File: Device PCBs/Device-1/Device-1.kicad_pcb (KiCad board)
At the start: 2 copper layers, 55 x 55 mm, 61 parts, among them J1 Conn_01x04_Female, J2 Conn_01x04_Female, U1 EBYTE_E32-433T20D, U10 signle_via, U11 signle_via, U12 signle_via, U13 signle_via, U14 signle_via, U15 signle_via, U16 signle_via, U17 signle_via, U18 signle_via, U19 signle_via, U2 MAX487E, U20 signle_via, U21 signle_via, U22 signle_via, U23 signle_via, U3 signle_via, U4 signle_via, U5 signle_via, U6 signle_via, U7 signle_via, U8 signle_via, U9 signle_via

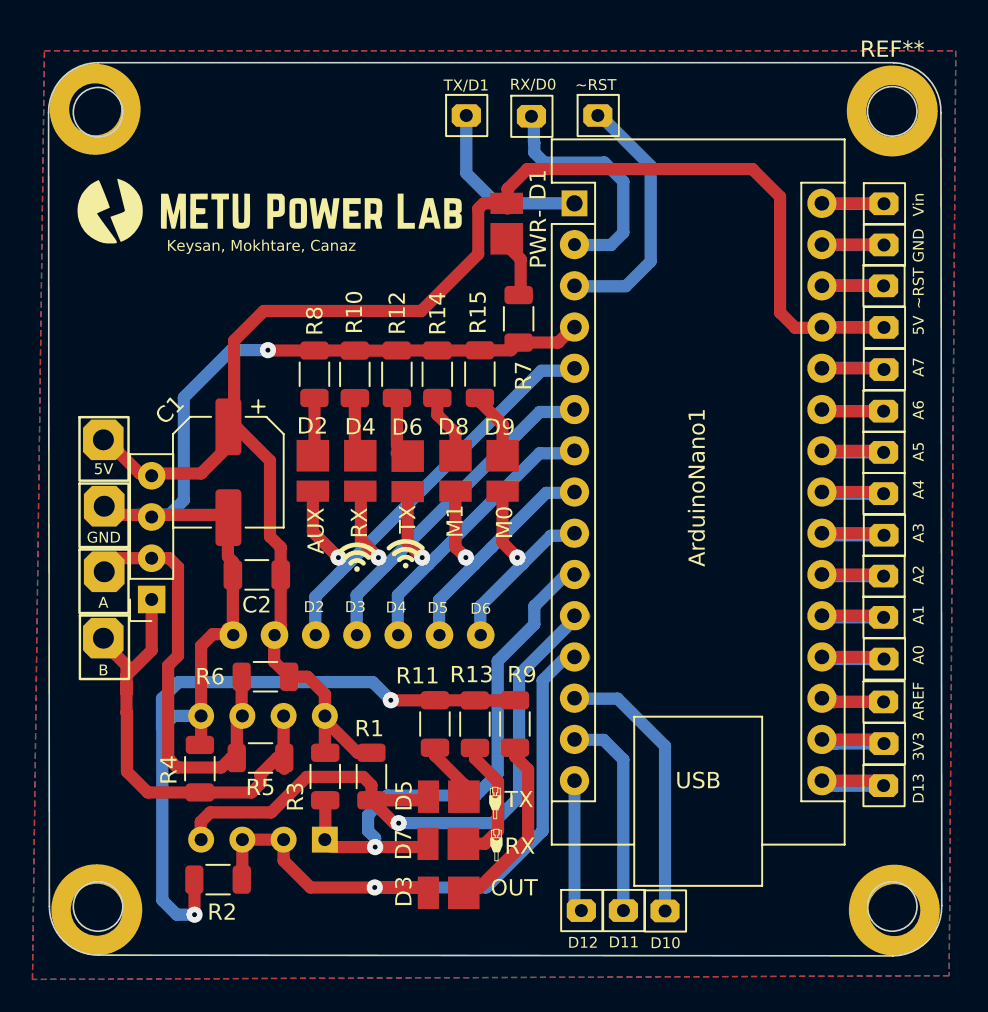
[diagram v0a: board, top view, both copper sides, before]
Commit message: PCBway gerbers are finished.
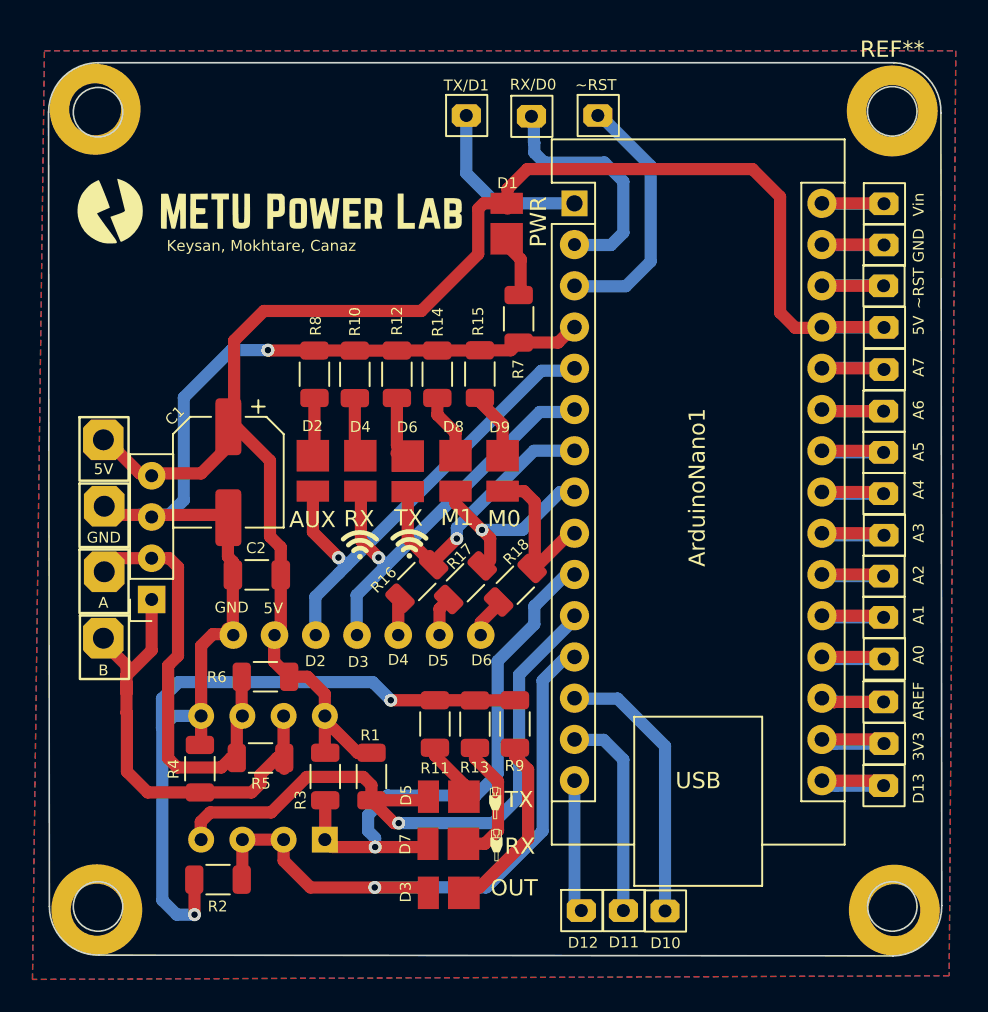
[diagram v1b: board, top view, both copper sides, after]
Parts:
- added R16: 3.3k, Resistor_SMD:R_1206_3216Metric, F.Cu at (35.6, 44.9)
- added R17: 3.3k, Resistor_SMD:R_1206_3216Metric, F.Cu at (38.6, 45.0)
- added R18: 3.3k, Resistor_SMD:R_1206_3216Metric, F.Cu at (41.7, 45.1)
- moved G*** 0.78 mm to (32.1, 42.7)
- moved G*** 0.64 mm to (35.2, 42.7)
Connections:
- ArduinoNano1 pad 7: EBYTE_RX -> Net-(ArduinoNano1-Pad7)
- ArduinoNano1 pad 8: M1 -> Net-(ArduinoNano1-Pad8)
- ArduinoNano1 pad 9: M0 -> Net-(ArduinoNano1-Pad9)
- D6 pad 2: EBYTE_RX -> Net-(ArduinoNano1-Pad7)
- D8 pad 2: M1 -> Net-(ArduinoNano1-Pad8)
- D9 pad 2: M0 -> Net-(ArduinoNano1-Pad9)
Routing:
- net EBYTE_RX: track 22.2 -> 2.32 mm, vias 1 -> 0
- net Net-(ArduinoNano1-Pad7): track 0.00 -> 17.4 mm, vias 0 -> 1
- net M1: track 18.2 -> 2.46 mm, vias 1 -> 0
- net M0: track 14.6 -> 2.64 mm, vias 1 -> 0
- net Net-(ArduinoNano1-Pad8): track 0.00 -> 11.8 mm, vias 0 -> 1
- net Net-(ArduinoNano1-Pad9): track 0.00 -> 9.76 mm
- net RS485_SS_RX_PIN: track 35.4 -> 34.2 mm
- net RS485_OUTPUT_ENABLE_PIN: track 40.2 -> 39.0 mm
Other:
- board text added: "PWR"
- board text removed: "PWR-"
